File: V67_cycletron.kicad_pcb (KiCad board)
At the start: 4 copper layers, 101.9 x 49.8 mm, 33 parts, among them J1 USB_C_Receptacle_USB2.0_16P, J3 Screw_Terminal_01x11, U1 LM1117DT-5.0, U2 LM1117DT-3.3, U4 ESP32-S3-WROOM-1

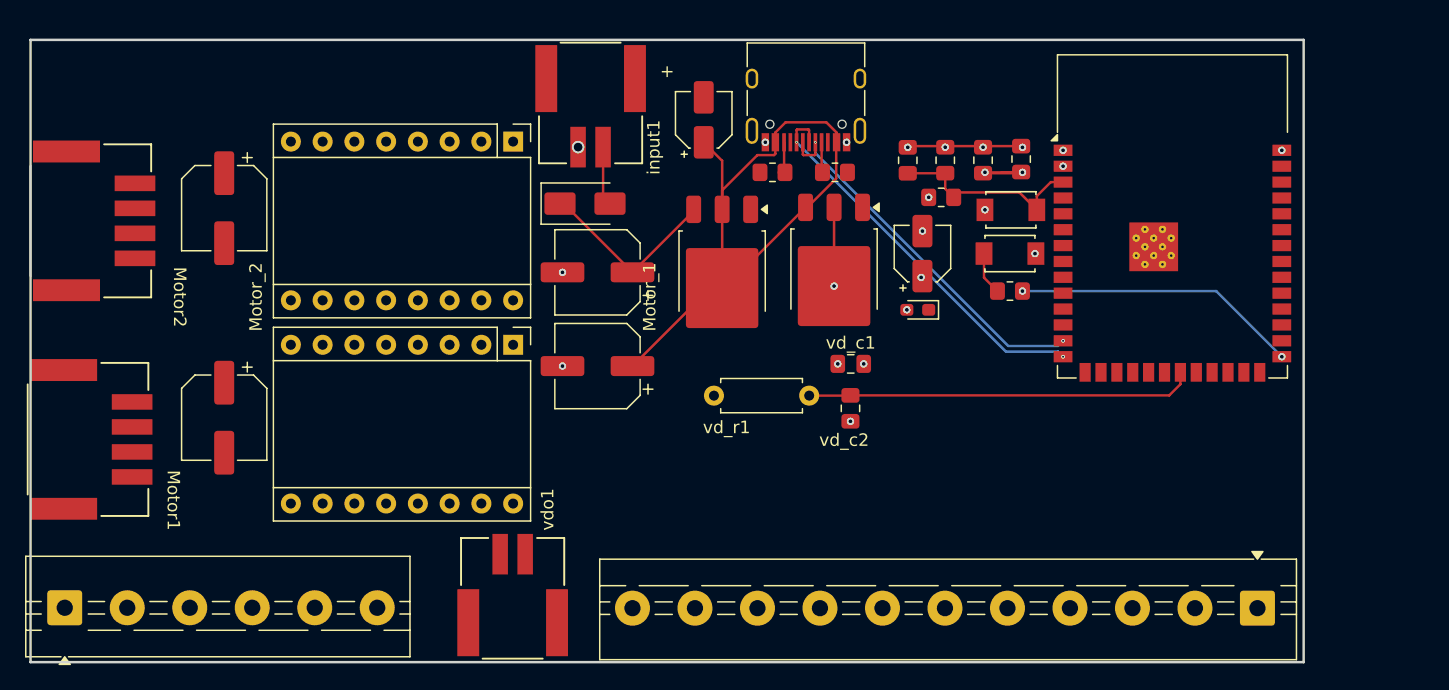
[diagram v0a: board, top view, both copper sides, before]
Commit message: progress so far, believe I just need to ensure manufacture compatibility
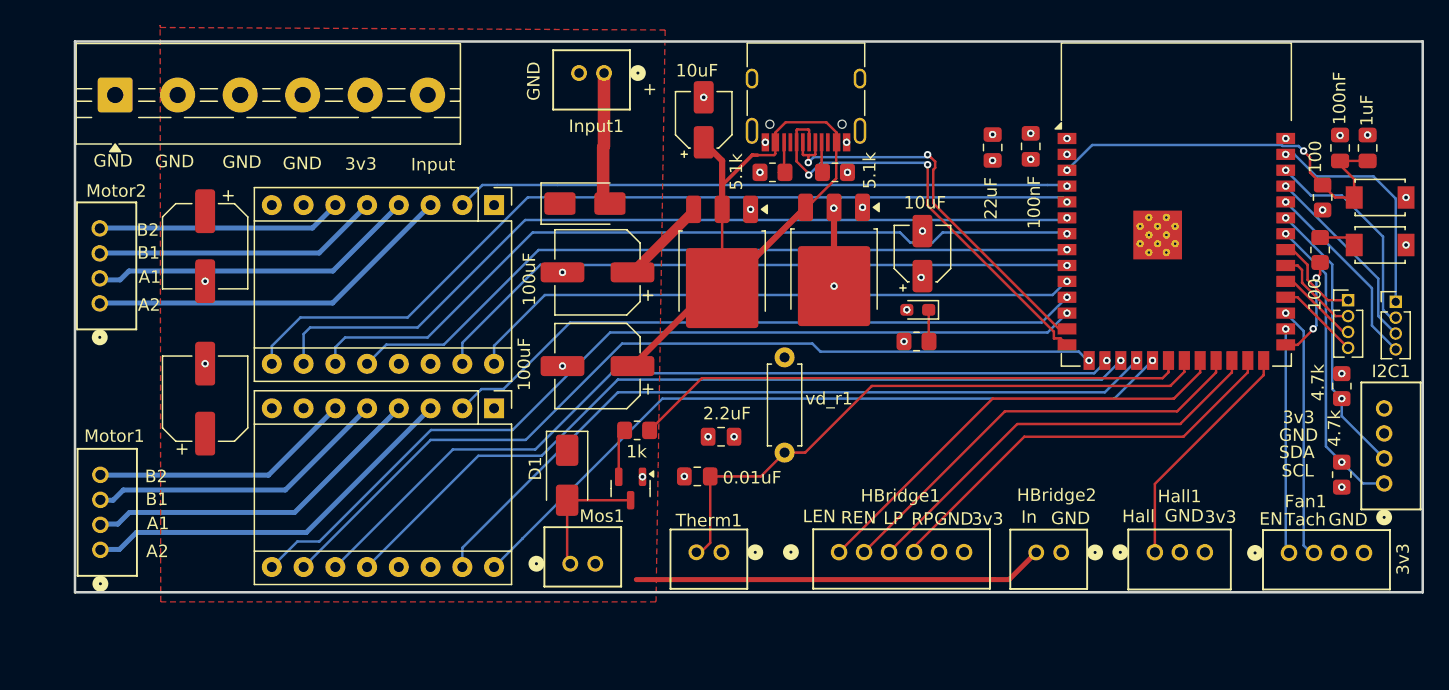
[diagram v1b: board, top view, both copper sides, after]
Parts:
- removed vdo1: 5023520200, Connector_4:CONN_SD-502352-001_02_MOL
- added D1: D_Schottky, Diode_SMD:D_SMA, F.Cu at (79.8, 107.2)
- added Fan1: PC_Fan, connector_4_vert:CONN4_B4B-PH_JST, F.Cu at (137.5, 113.4)
- added HBridge1: B6B-PH-K-S, connector_6_vert:CONN_B6B-PH-K-S_JST, F.Cu at (101.5, 113.4)
- added HBridge2: B2B-PH-K-S, connector_2_vert:CONN2_B2B-PH-K-S_JST, F.Cu at (119.3, 113.4)
- added Hall1: Hall_Sens, connector_3_vert:CONN_B3B-PH-K-SLFSN_JST, F.Cu at (126.8, 113.4)
- added I2C1: MCP9600, connector_4_vert:CONN4_B4B-PH_JST, F.Cu at (145.1, 107.9)
- added J2: Conn_01x04_Socket, Connector_PinHeader_1.27mm:PinHeader_1x04_P1.27mm_Vertical, F.Cu at (146.1, 93.3)
- added Mos1: B2B-PH-K-S, connector_2_vert:CONN2_B2B-PH-K-S_JST, F.Cu at (80.0, 114.3)
- added R3: 1k, Resistor_SMD:R_0805_2012Metric_Pad1.20x1.40mm_HandSolder, F.Cu at (107.7, 96.5)
- added R4: 4.7k, Resistor_SMD:R_0805_2012Metric_Pad1.20x1.40mm_HandSolder, F.Cu at (141.7, 107.2)
- added R5: 4.7k, Resistor_SMD:R_0805_2012Metric_Pad1.20x1.40mm_HandSolder, F.Cu at (141.7, 100.1)
- added Therm1: B2B-PH-K-S, connector_2_vert:CONN2_B2B-PH-K-S_JST, F.Cu at (92.1, 113.4)
- added mosfet4: HD2305, Package_TO_SOT_SMD:SOT-23, F.Cu at (84.8, 108.3)
- added tr3: 1k, Resistor_SMD:R_0805_2012Metric_Pad1.20x1.40mm_HandSolder, F.Cu at (85.4, 103.6)
- Input1: renamed from input1; value 5023520200 -> B2B-PH-K-S; footprint Connector_4:CONN_SD-502352-001_02_MOL -> connector_2_vert:CONN2_B2B-PH-K-S_JST
- J3: value Screw_Terminal_01x11 -> Conn_01x04_Socket; footprint TerminalBlock:TerminalBlock_MaiXu_MX126-5.0-11P_1x11_P5.00mm -> Connector_PinHeader_1.27mm:PinHeader_1x04_P1.27mm_Vertical
- Motor1: value 5023520400 -> Motor1; footprint Connector_4:CONN_SD-502352-001_04_MOL -> connector_4_vert:CONN4_B4B-PH_JST
- Motor2: value 5023520400 -> Motor2; footprint Connector_4:CONN_SD-502352-001_04_MOL -> connector_4_vert:CONN4_B4B-PH_JST
- moved Rails1 41.2 mm to (43.6, 76.8)
- moved C2 34.6 mm to (141.6, 81.0)
- moved C1 33.8 mm to (143.8, 81.0)
- moved R_En1 30.5 mm to (140.2, 85.0), turned to 90 degrees
- moved Boot1 29.6 mm to (144.8, 88.8)
- moved En1 29.6 mm to (144.8, 85.0), turned to 0 degrees
- moved J3 25.7 mm to (142.2, 93.2), turned to 0 degrees
- moved R_boot1 25.0 mm to (140.0, 89.2), turned to -90 degrees
- moved vd_c2 13.4 mm to (90.2, 107.3), turned to 180 degrees
- moved vd_c1 11.9 mm to (92.1, 104.1)
- moved Motor1 8.89 mm to (42.4, 113.2), turned to 90 degrees
- moved Motor2 6.64 mm to (42.4, 93.5), turned to 90 degrees
- moved Motor_1 5.30 mm to (73.9, 101.9)
- moved Motor_2 5.30 mm to (73.9, 85.6)
- moved vd_r1 4.97 mm to (97.2, 105.4), turned to 90 degrees
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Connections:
- J3 pad 1: I20 -> IO40
- J3 pad 2: I19 -> IO39
- J3 pad 3: I18 -> IO38
- J3 pad 4: I17 -> IO37
- Motor1 pad 1: Motor1_A1 -> Motor1_A2
- Motor1 pad 2: Motor1_A2 -> Motor1_A1
- Motor1 pad 3: Motor1_B2 -> Motor1_B1
- Motor1 pad 4: Motor1_B1 -> Motor1_B2
- Motor2 pad 3: Motor2_B2 -> Motor2_B1
- Motor2 pad 4: Motor2_B1 -> Motor2_B2
- U4 pad 10: I10 -> Motor2_DIR
- U4 pad 11: I11 -> Motor1_FLT
- U4 pad 12: I12 -> Motor1_EN
- U4 pad 15: I15 -> Motor1_M0
- U4 pad 16: I16 -> Motor1_M1
- U4 pad 17: I17 -> Motor1_M2
- U4 pad 18: I18 -> Motor1_STEP
- U4 pad 19: I19 -> Motor1_DIR
- U4 pad 20: I20 -> mosfet1_i
- U4 pad 22: mosfet1_i -> L_EN
- U4 pad 23: mosfet2_i -> R_EN
- U4 pad 24: mosfet3_i -> LPWM
- U4 pad 25: Motor1_FLT -> RPWM
- U4 pad 26: Motor1_EN -> Hall_i
- U4 pad 28: Motor1_M0 -> FAN_En_o
- U4 pad 29: Motor1_M1 -> FAN_Tach_i
- U4 pad 30: Motor1_M2 -> IO37
- U4 pad 31: Motor1_STEP -> IO38
- U4 pad 32: Motor1_DIR -> IO39
- U4 pad 33: Motor2_EN -> IO40
- U4 pad 34: Motor2_FLT -> SCL
- U4 pad 35: Motor2_M0 -> SDA
- U4 pad 36: Motor2_M1 -> RX
- U4 pad 37: Motor2_M2 -> TX
- U4 pad 38: Motor2_STEP -> IO2
- U4 pad 39: Motor2_DIR -> IO1
- U4 pad 4: IO4 -> Motor2_FLT
- U4 pad 5: IO5 -> Motor2_EN
- U4 pad 6: IO6 -> Motor2_M0
- U4 pad 7: IO7 -> Motor2_M1
- U4 pad 8: I08 -> Motor2_M2
- U4 pad 9: I09 -> Motor2_STEP
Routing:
- net Motor1_EN: track 0.00 -> 72.0 mm, vias 0 -> 1
- net Motor1_M0: track 0.00 -> 70.7 mm, vias 0 -> 1
- net Motor2_EN: track 0.00 -> 70.2 mm, vias 0 -> 1
- net Motor1_M1: track 0.00 -> 68.6 mm, vias 0 -> 1
- net Motor2_M0: track 0.00 -> 67.6 mm, vias 0 -> 1
- net Motor1_M2: track 0.00 -> 67.1 mm, vias 0 -> 1
- net Motor2_M1: track 0.00 -> 64.4 mm, vias 0 -> 1
- net Motor1_STEP: track 0.00 -> 61.7 mm, vias 0 -> 1
- net Motor2_M2: track 0.00 -> 59.8 mm, vias 0 -> 1
- net Motor1_DIR: track 0.00 -> 59.5 mm, vias 0 -> 1
- net Motor2_STEP: track 0.00 -> 52.7 mm, vias 0 -> 1
- net Motor1_FLT: track 0.00 -> 52.1 mm, vias 0 -> 1
- net Motor2_DIR: track 0.00 -> 49.5 mm, vias 0 -> 1
- net Motor2_FLT: track 0.00 -> 49.1 mm, vias 0 -> 1
- net mosfet1_i: track 0.00 -> 44.4 mm
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- added copper zone on F.Cu, net +12V
- added copper zone on In1.Cu, net 3V3
- added copper zone on In2.Cu, net GND
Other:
- board size 101.9 x 49.8 mm -> 107.8 x 44.1 mm
- board text added: "0.01uF"
- board text added: "100"
- board text added: "100nF"
- board text added: "100uF"
- board text added: "10uF"
- board text added: "1k"
- board text added: "1uF"
- board text added: "2.2uF"
- board text added: "22uF"
- board text added: "3v3"
- board text added: "4.7k"
- board text added: "5.1k"
- board text added: "A1"
- board text added: "A2"
- board text added: "B1"
- board text added: "B2"
- board text added: "EN"
- board text added: "GND"
- board text added: "Hall"
- board text added: "In"
- board text added: "Input"
- board text added: "LEN"
- board text added: "LP"
- board text added: "REN"
- board text added: "RP"
- board text added: "SCL"
- board text added: "SDA"
- board text added: "Tach"
